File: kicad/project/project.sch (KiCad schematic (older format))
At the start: 47 parts, among them J1 SWD, J3 Voltmeter, Q1 Si2319CDS, Q2 2N7002, U1 ADS1015, U2 AP7380, U3 STM32L031F4Px, U4 VN7003ALH

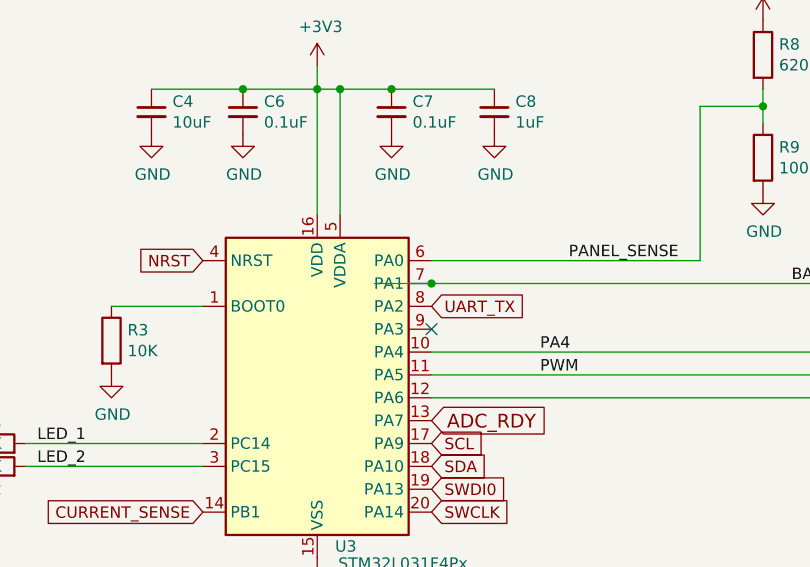
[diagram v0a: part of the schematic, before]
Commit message: Tuning
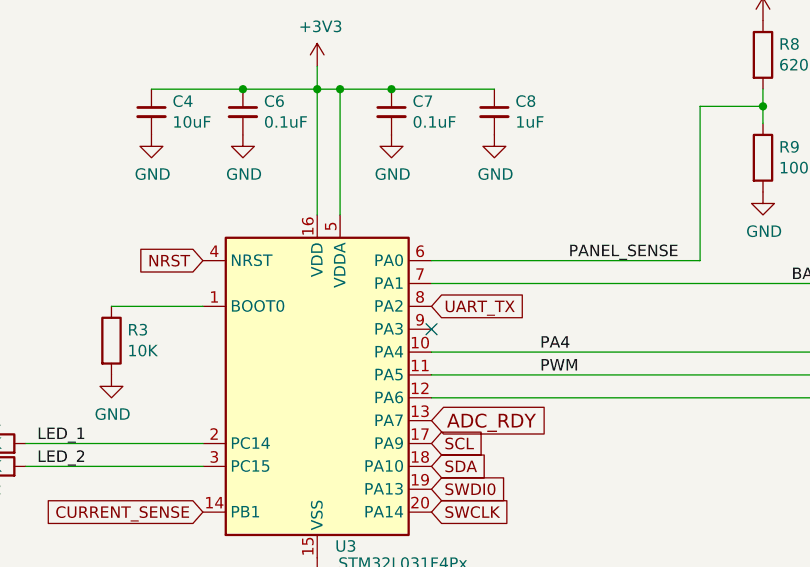
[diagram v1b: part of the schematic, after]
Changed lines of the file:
@@
 	1400 7275 1400 7125
-Wire Wire Line
-	4300 3925 4550 3925
 Wire Wire Line
 	6000 3075 6000 3150
@@
 	0    -1   -1   0
 $EndComp
-Connection ~ 4550 3925
-Wire Wire Line
-	4550 3925 6650 3925
 Wire Wire Line
 	6850 4225 6850 4075
@@
 	9925 2975 9825 2975
 Connection ~ 9825 2975
+Wire Wire Line
+	4550 3925 6650 3925
 $EndSCHEMATC

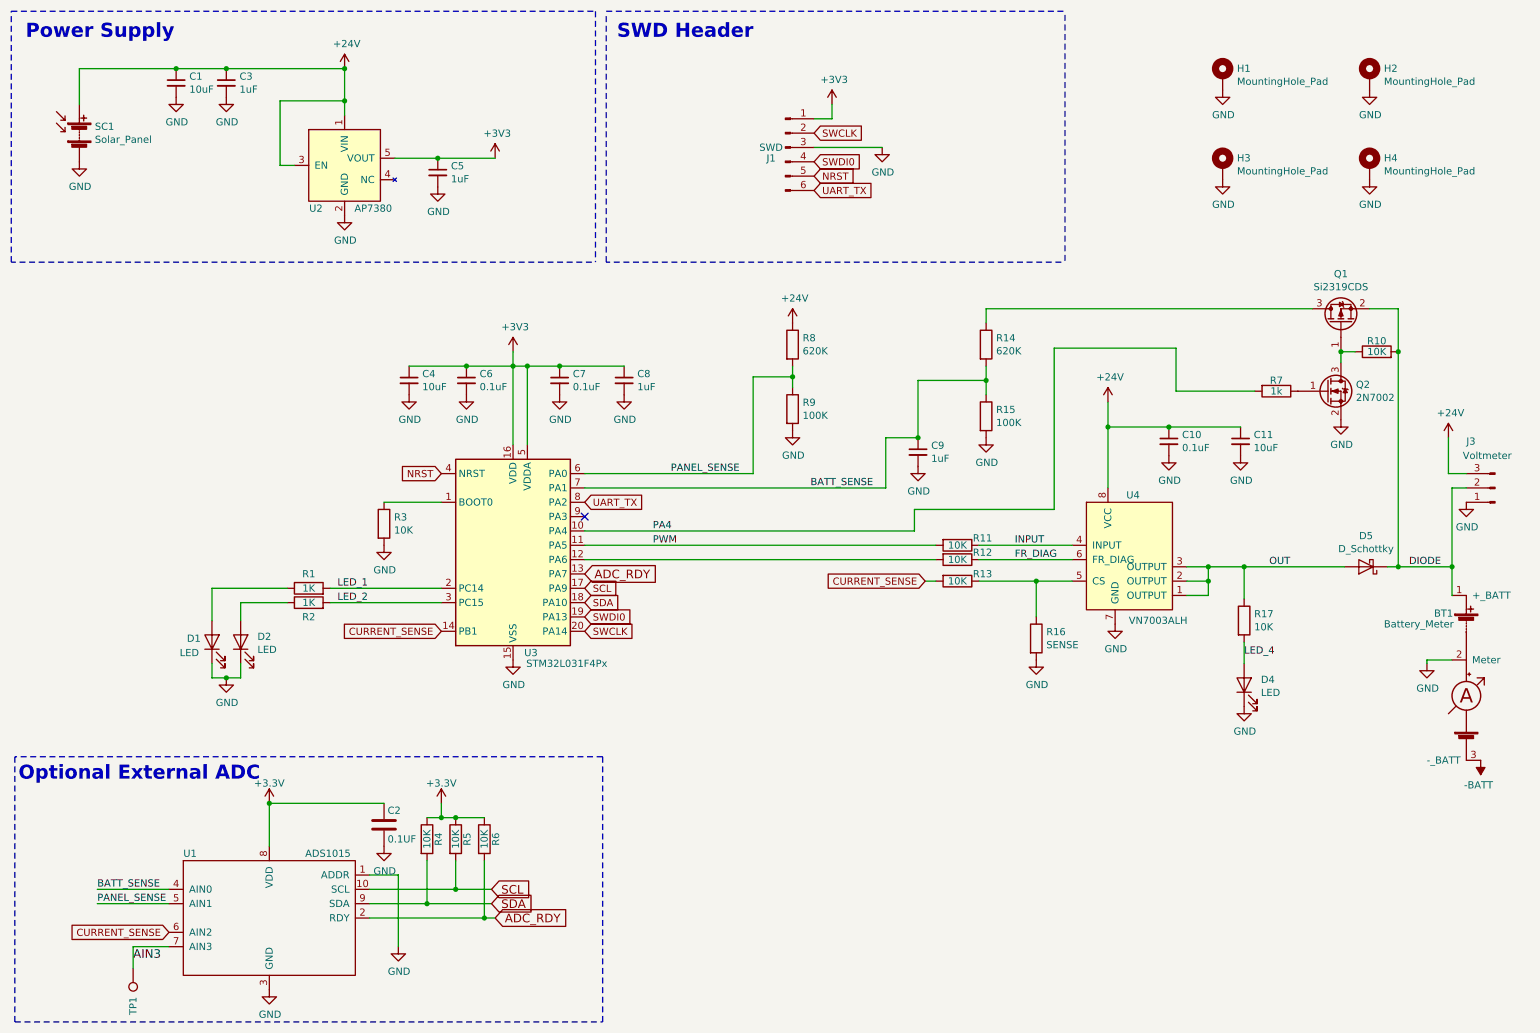
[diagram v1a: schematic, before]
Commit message: VN7004CLHTR
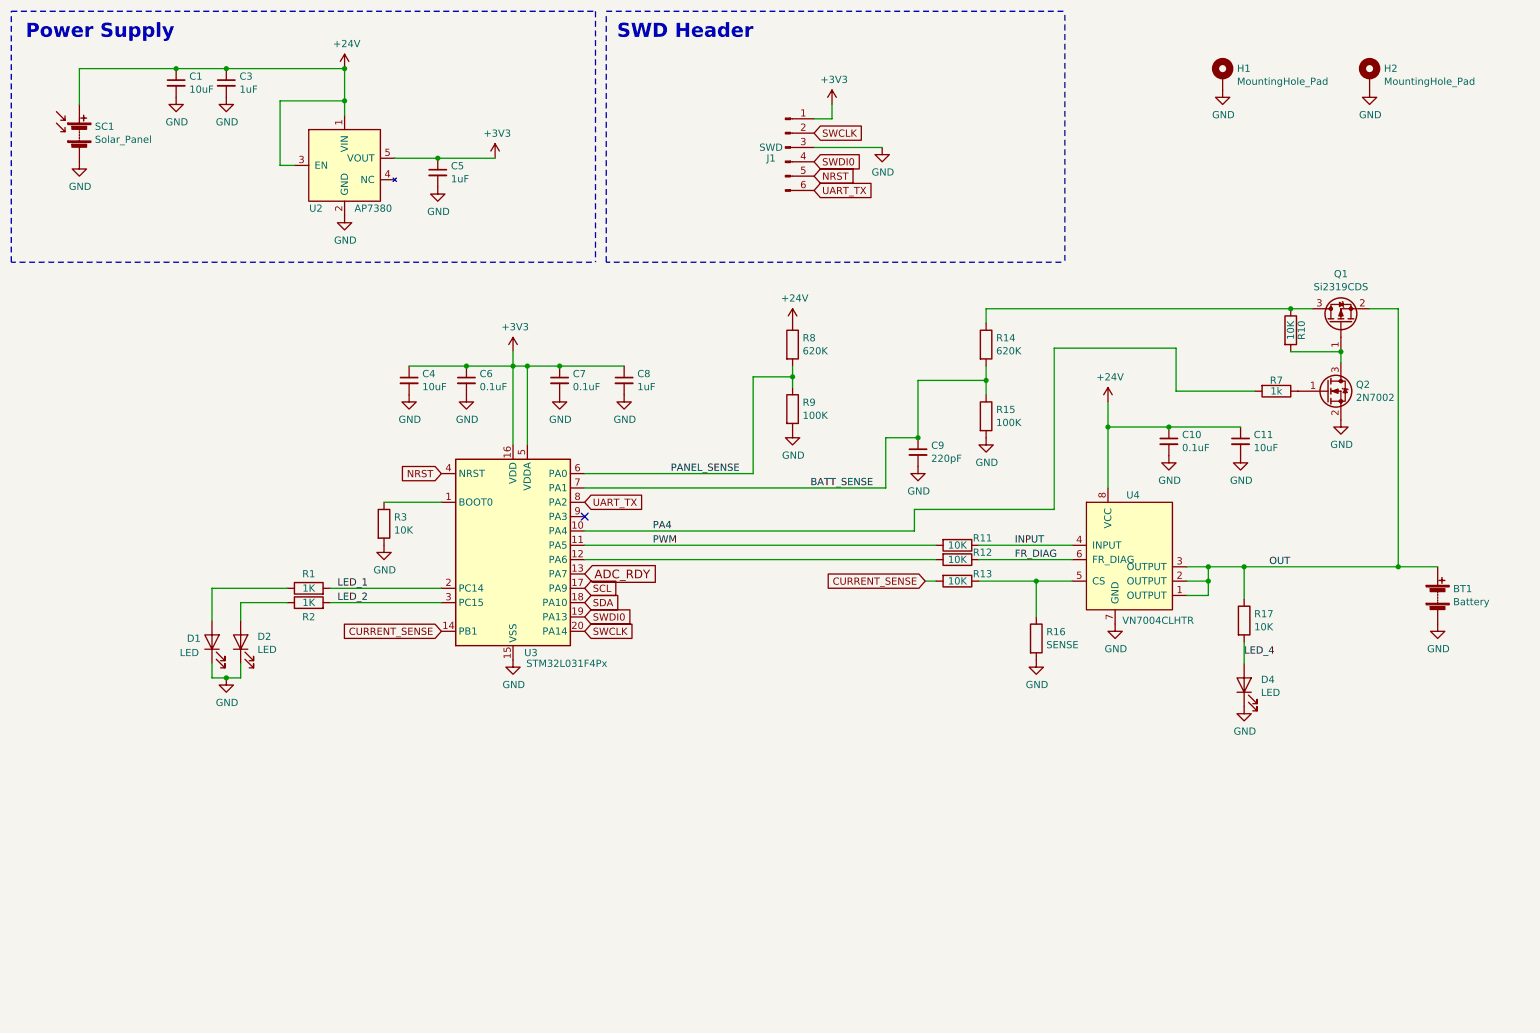
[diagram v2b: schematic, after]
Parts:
- removed BT1: Battery_Meter, theapi:TerminalBlock_Meter, symbol theapi_Battery:Battery_Meter
- removed C2: 0.1UF, Capacitor_SMD:C_0603_1608Metric_Pad1.05x0.95mm_HandSolder, symbol project-rescue:C-stm32l053c-rescue
- removed D5: D_Schottky, Diode_THT:D_DO-201AD_P12.70mm_Horizontal, symbol Device:D_Schottky
- removed H3, H4: MountingHole_Pad, MountingHole:MountingHole_3.2mm_M3_Pad, symbol Mechanical:MountingHole_Pad
- removed J3: Voltmeter, theapi:Voltmeter_Header_1x03, symbol Connector:Conn_01x03_Male
- removed R4, R5, R6: 10K, Resistor_SMD:R_0603_1608Metric_Pad1.05x0.95mm_HandSolder, symbol project-rescue:R-stm32l053c-rescue
- removed TP1: TestPoint, TestPoint:TestPoint_Pad_D1.0mm, symbol Connector:TestPoint
- removed U1: ADS1015, theapi:TSSOP-10_3x3mm_P0.5mm, symbol project-rescue:ADS1015-adc
- added BT1: Battery, TerminalBlock:TerminalBlock_bornier-2_P5.08mm, symbol Device:Battery
- C9: value 1uF -> 220pF
- U4: value VN7003ALH -> VN7004CLHTR
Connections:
- net GND: now also BT1.2 (-)
- net OUT: now also Q1.2 (S), BT1.1 (+)
- net at Q1.3 (D), R14.1: now also R10.1
- net at Q1.1 (G), Q2.3 (D): now also R10.2; no longer R10.1
- removed net DIODE: Q1.2 (S), R10.2
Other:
- note removed: "Optional External ADC"
- moved on the sheet: R10

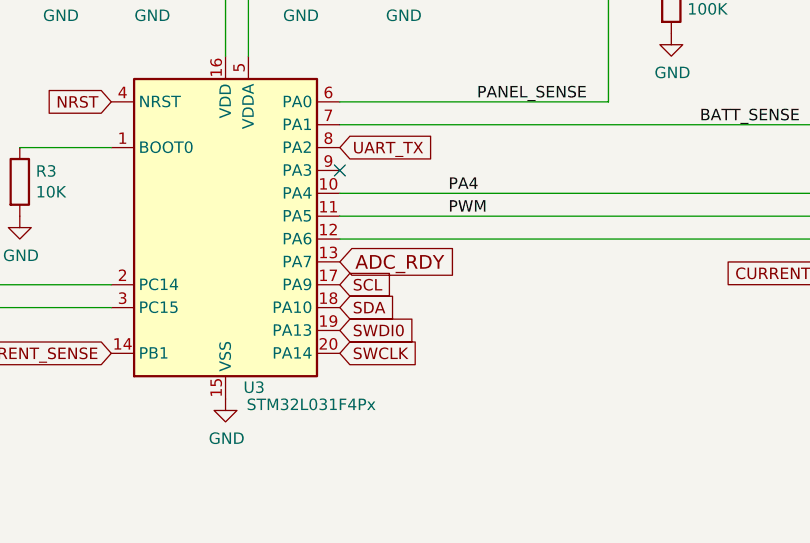
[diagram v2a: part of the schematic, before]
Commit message: VN7004CLHTR
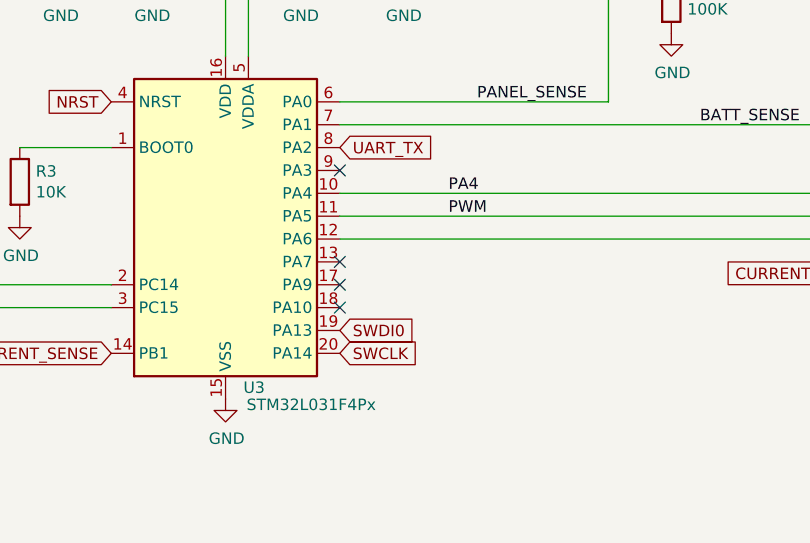
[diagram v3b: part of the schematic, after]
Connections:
- net ADC_RDY: no longer names the net of U3.13 (PA7)
- net SCL: no longer names the net of U3.17 (PA9)
- net SDA: no longer names the net of U3.18 (PA10)
- no-connect marks 1 -> 4
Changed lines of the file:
@@
 	1    0    0    -1
 $EndComp
-Text GLabel 4550 4625 2    50   Input ~ 0
-SCL
-Text GLabel 4550 4725 2    50   Input ~ 0
-SDA
 Text GLabel 3550 4925 0    50   Input ~ 0
 CURRENT_SENSE
@@
 Text GLabel 6150 1850 2    50   Input ~ 0
 UART_TX
-Text GLabel 4550 4525 2    60   Input ~ 0
-ADC_RDY
 Wire Wire Line
 	6000 3075 6000 3150
@@
 Wire Wire Line
 	10225 2675 10225 4475
+NoConn ~ 4550 4625
+NoConn ~ 4550 4525
+NoConn ~ 4550 4725
 $EndSCHEMATC
